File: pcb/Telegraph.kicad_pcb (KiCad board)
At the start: 2 copper layers, 87 x 88 mm, 187 parts, among them Q1 BC848, Q10 BC848, Q11 BC848, Q14 MMBT2222, Q2 BC848, Q5 DVIUC6-4SC6, Q6 BC848, Q7 BC848, SW1 DIPx4, SW2 SWITCH_H, SW3 BUTTON, SW4 SWITCH_2x, SW5 SWITCH_2x, U1 L6470, U2 L6470

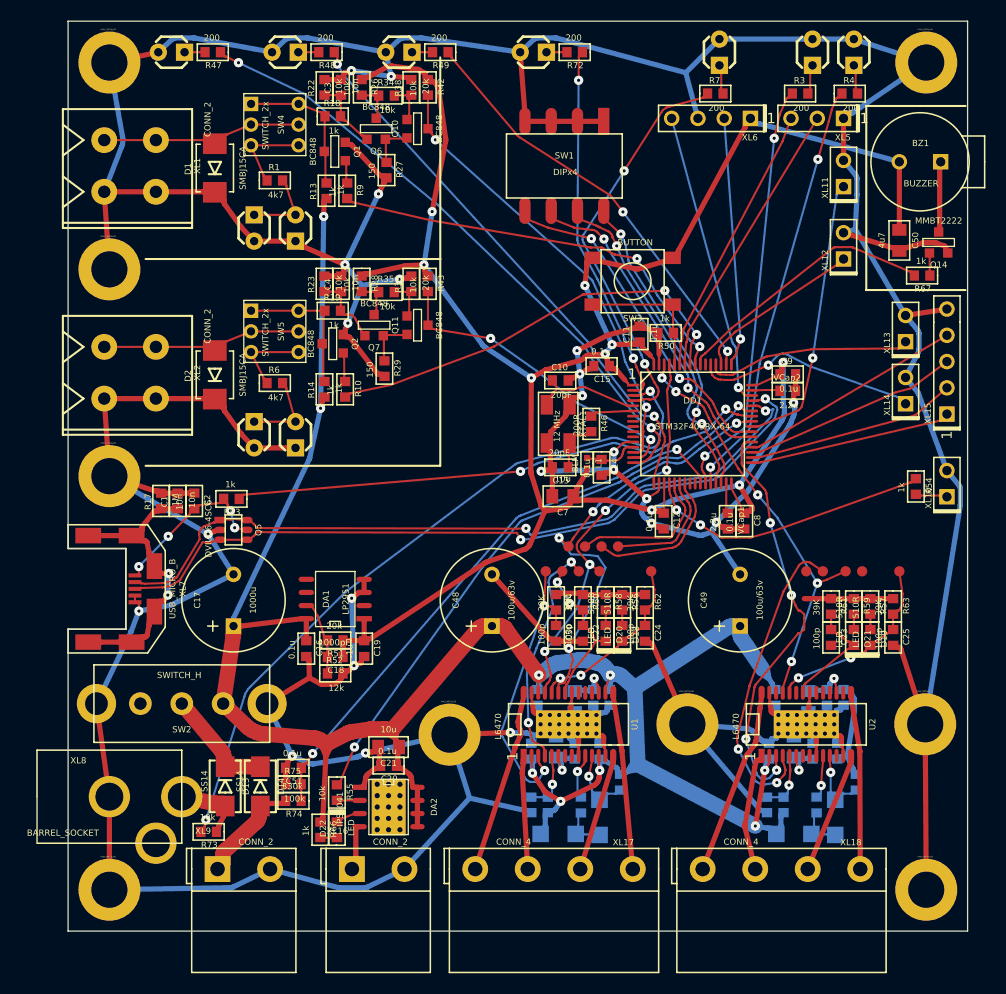
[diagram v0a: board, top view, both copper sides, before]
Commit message: Proceeding
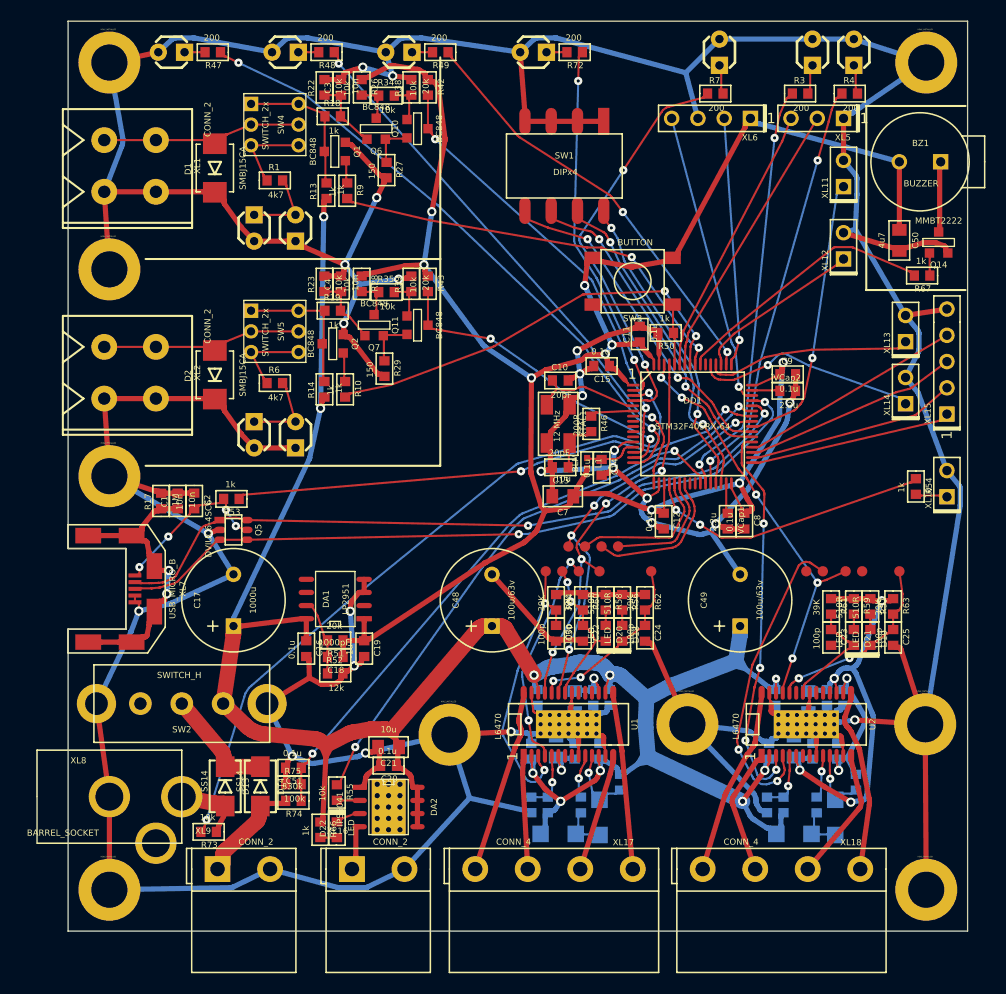
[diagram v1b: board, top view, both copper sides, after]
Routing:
- net /Vdd2: track 17.9 -> 45.3 mm, vias 2 -> 4
- net GND: track 698.5 -> 707.9 mm, vias 23 -> 24
- net +12V: track 229.9 -> 235.4 mm, vias 9 -> 12
- net /MOTOR_CS: track 43.1 -> 38.9 mm
- net /D-: track 72.5 -> 69.2 mm
- net /STBY/RST: track 68.7 -> 65.9 mm
- net /D+: track 72.7 -> 70.0 mm
- net /OUT2_1B: track 11.8 -> 13.0 mm
- net /OUT2_1A: track 11.6 -> 12.4 mm
- net /PwrSrcSns: track 70.1 -> 69.5 mm
- net /OUT2_2B: track 17.1 -> 17.7 mm
- net /DS2: track 32.4 -> 31.8 mm
- net /BUSY/SYNC_1: track 15.4 -> 14.9 mm
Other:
- net class Wide: via_dia 1 -> 0.9; via_drill 0.5 -> 0.4
